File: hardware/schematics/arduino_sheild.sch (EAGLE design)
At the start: 37 parts, among them IC3 LM358, Q1 IRL520N-H, Q2 IRL520N-H, Q3 IRF9Z24, Q4 IRL520N-H, Q5 IRL520N-H, Q6 IRF9Z24, X5 STEREOJACK, X6 STEREOJACK

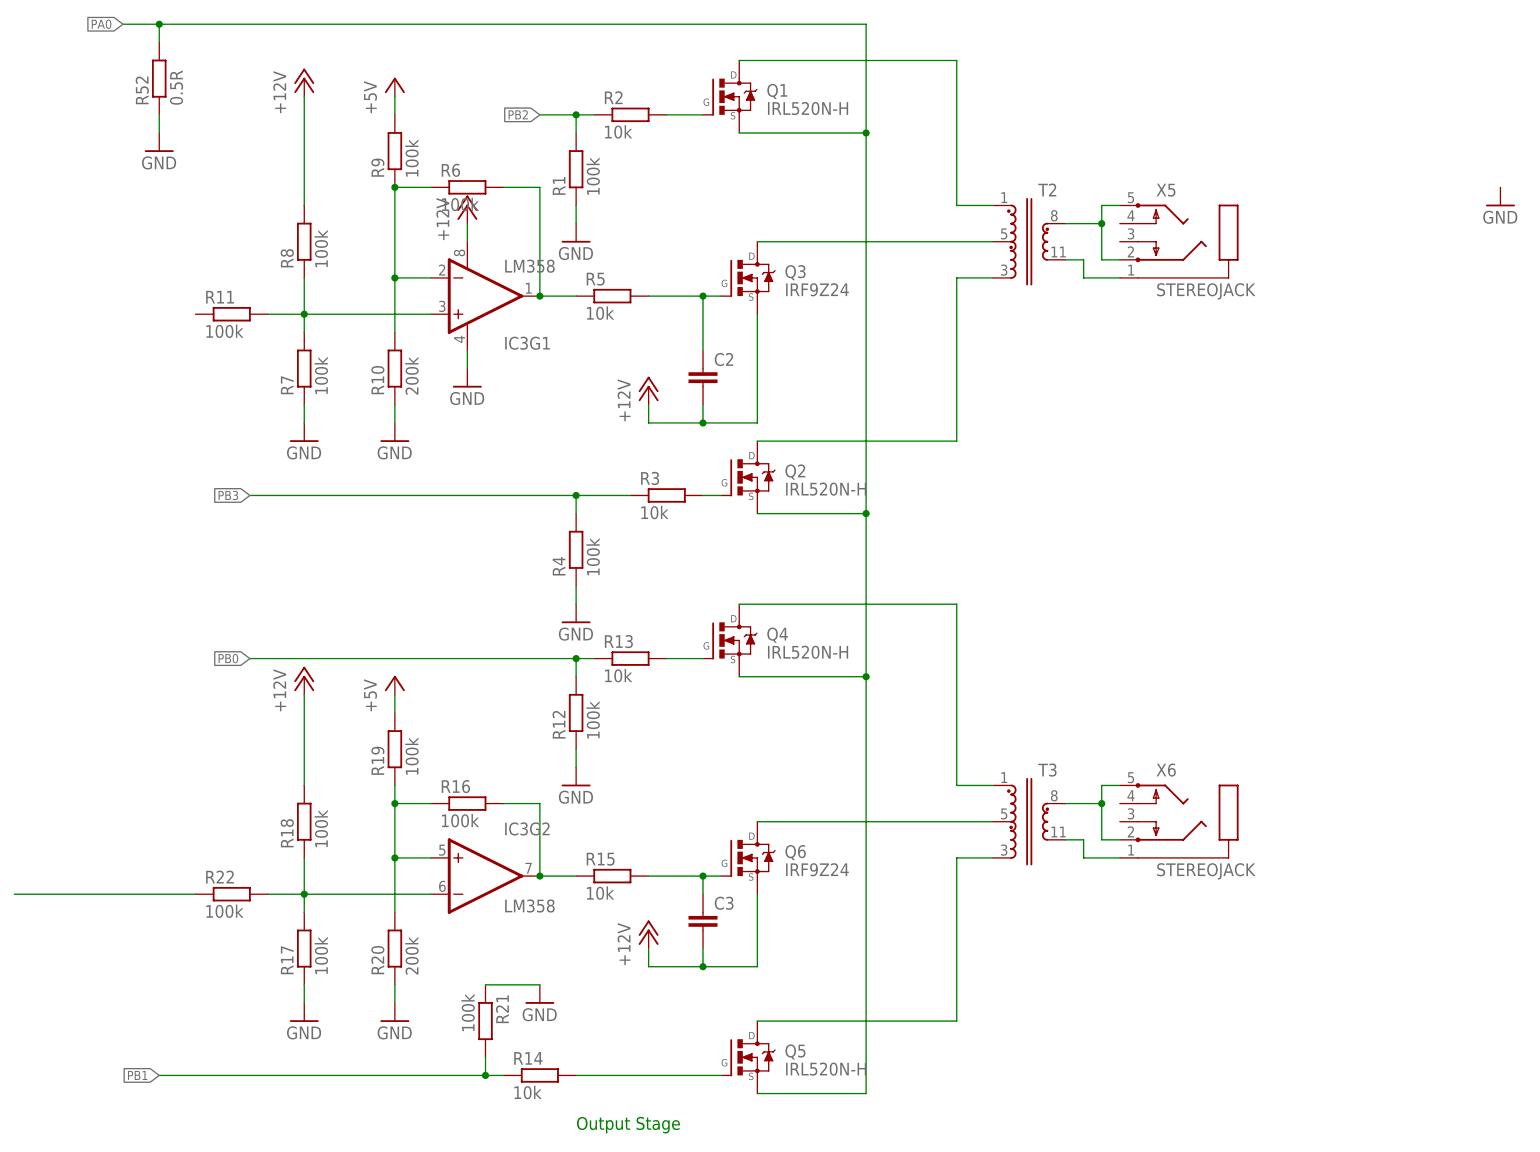
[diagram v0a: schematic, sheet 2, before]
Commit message: Schematics
WIP
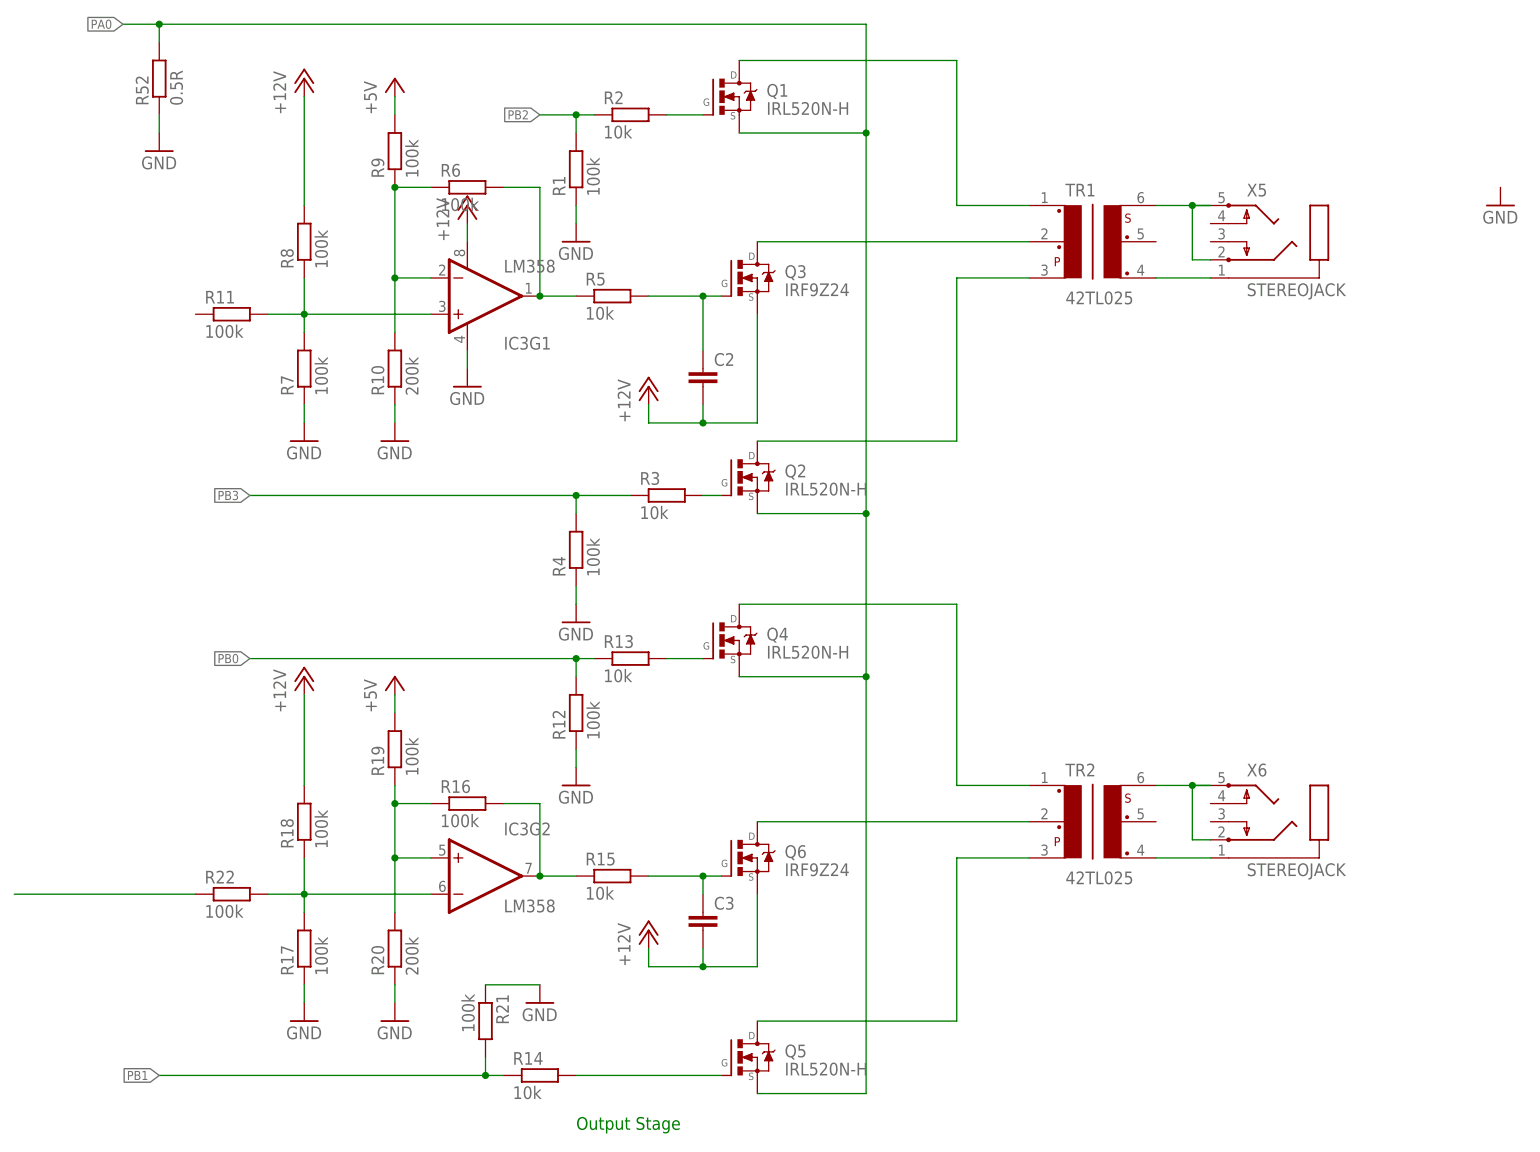
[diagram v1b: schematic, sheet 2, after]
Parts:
- removed T2, T3: (no value), Eagle_POWER_MAGNETICS_rev16b:WE-FB_LT35XX/LT3748_EFD25_750310988
- added TR1, TR2: 42TL025, trafo-xicon:42TL025
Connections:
- removed net N$66: T3.3, X6.1
- removed net N$67: T3.2, X6.2, X6.5
- removed net N$77: T2.3, X5.1
- removed net N$78: T2.2, X5.2, X5.5
- new net N$1: TR1.4, X5.1
- new net N$2: TR1.6, X5.2, X5.5
- new net N$3: TR2.6, X6.2, X6.5
- new net N$4: TR2.4, X6.1
- net N$34: now also TR1.1; no longer T2.1
- net N$35: now also TR1.2; no longer T2.5
- net N$36: now also TR2.1; no longer T3.1
- net N$37: now also TR2.2; no longer T3.5
- net N$38: now also TR2.3; no longer T3.4
- net N$39: now also TR1.3; no longer T2.4
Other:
- moved on the sheet: X5, X6
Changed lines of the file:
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@@
 <part name="R52" library="eagle-ltspice" deviceset="R" device="0207/10" value="0.5R"/>
 <part name="GND21" library="supply1" deviceset="GND" device=""/>
-<part name="T2" library="Eagle_POWER_MAGNETICS_rev16b" deviceset="WE-FB_LT35XX/LT3748_EFD25_750310988" device=""/>
-<part name="T3" library="Eagle_POWER_MAGNETICS_rev16b" deviceset="WE-FB_LT35XX/LT3748_EFD25_750310988" device=""/>
 <part name="U$3" library="adafruit" deviceset="ARDUINO" device="UNO"/>
 <part name="GND40" library="supply1" deviceset="GND" device=""/>
@@
 <part name="P+8" library="supply1" deviceset="+12V" device=""/>
 <part name="P+9" library="supply1" deviceset="+12V" device=""/>
+<part name="TR1" library="trafo-xicon" deviceset="42T?*" device="L" technology="025"/>
+<part name="TR2" library="trafo-xicon" deviceset="42T?*" device="L" technology="025"/>
 </parts>
 <sheets>
@@
 <instance part="R22" gate="G$1" x="50.8" y="40.64"/>
 <instance part="FRAME6" gate="G$1" x="0" y="0"/>
-<instance part="X5" gate="1" x="187.96" y="134.62"/>
-<instance part="X6" gate="1" x="187.96" y="53.34"/>
+<instance part="X5" gate="1" x="200.66" y="134.62"/>
+<instance part="X6" gate="1" x="200.66" y="53.34"/>
 <instance part="R52" gate="G$1" x="40.64" y="154.94" rot="R90"/>
 <instance part="GND21" gate="1" x="40.64" y="144.78"/>
-<instance part="T2" gate="G$1" x="162.56" y="132.08"/>
-<instance part="T3" gate="G$1" x="162.56" y="50.8"/>
 <instance part="GND42" gate="1" x="228.6" y="137.16"/>
 <instance part="P+7" gate="1" x="73.66" y="71.12"/>
@@
 <instance part="P+8" gate="1" x="109.22" y="111.76"/>
 <instance part="P+9" gate="1" x="109.22" y="35.56"/>
+<instance part="TR1" gate="G$1" x="170.18" y="132.08"/>
+<instance part="TR2" gate="G$1" x="170.18" y="50.8"/>
 </instances>
 <busses>
@@
 <wire x1="121.92" y1="157.48" x2="152.4" y2="157.48" width="0.1524" layer="91"/>
 <wire x1="152.4" y1="157.48" x2="152.4" y2="137.16" width="0.1524" layer="91"/>
-<wire x1="157.48" y1="137.16" x2="152.4" y2="137.16" width="0.1524" layer="91"/>
-<pinref part="T2" gate="G$1" pin="1"/>
+<pinref part="TR1" gate="G$1" pin="1"/>
+<wire x1="162.56" y1="137.16" x2="152.4" y2="137.16" width="0.1524" layer="91"/>
 </segment>
 </net>
@@
 <segment>
 <pinref part="Q3" gate="G$1" pin="D"/>
-<wire x1="124.46" y1="132.08" x2="157.48" y2="132.08" width="0.1524" layer="91"/>
-<pinref part="T2" gate="G$1" pin="5"/>
+<wire x1="124.46" y1="132.08" x2="162.56" y2="132.08" width="0.1524" layer="91"/>
+<pinref part="TR1" gate="G$1" pin="2"/>
 </segment>
 </net>
@@
 <wire x1="121.92" y1="81.28" x2="152.4" y2="81.28" width="0.1524" layer="91"/>
 <wire x1="152.4" y1="81.28" x2="152.4" y2="55.88" width="0.1524" layer="91"/>
-<wire x1="157.48" y1="55.88" x2="152.4" y2="55.88" width="0.1524" layer="91"/>
-<pinref part="T3" gate="G$1" pin="1"/>
+<pinref part="TR2" gate="G$1" pin="1"/>
+<wire x1="162.56" y1="55.88" x2="152.4" y2="55.88" width="0.1524" layer="91"/>
 </segment>
 </net>
@@
 <segment>
 <pinref part="Q6" gate="G$1" pin="D"/>
-<wire x1="124.46" y1="50.8" x2="157.48" y2="50.8" width="0.1524" layer="91"/>
-<pinref part="T3" gate="G$1" pin="5"/>
+<wire x1="124.46" y1="50.8" x2="162.56" y2="50.8" width="0.1524" layer="91"/>
+<pinref part="TR2" gate="G$1" pin="2"/>
 </segment>
 </net>
@@
 <wire x1="124.46" y1="22.86" x2="152.4" y2="22.86" width="0.1524" layer="91"/>
 <wire x1="152.4" y1="22.86" x2="152.4" y2="45.72" width="0.1524" layer="91"/>
-<wire x1="157.48" y1="45.72" x2="152.4" y2="45.72" width="0.1524" layer="91"/>
-<pinref part="T3" gate="G$1" pin="4"/>
+<pinref part="TR2" gate="G$1" pin="3"/>
+<wire x1="162.56" y1="45.72" x2="152.4" y2="45.72" width="0.1524" layer="91"/>
 </segment>
 </net>
@@
 <wire x1="124.46" y1="104.14" x2="152.4" y2="104.14" width="0.1524" layer="91"/>
 <wire x1="152.4" y1="104.14" x2="152.4" y2="127" width="0.1524" layer="91"/>
-<wire x1="157.48" y1="127" x2="152.4" y2="127" width="0.1524" layer="91"/>
-<pinref part="T2" gate="G$1" pin="4"/>
+<pinref part="TR1" gate="G$1" pin="3"/>
+<wire x1="162.56" y1="127" x2="152.4" y2="127" width="0.1524" layer="91"/>
 </segment>
 </net>
@@
 </segment>
 </net>
-<net name="N$66" class="0">
-<segment>
-<pinref part="X6" gate="1" pin="1"/>
-<wire x1="175.26" y1="45.72" x2="170.18" y2="45.72" width="0.1524" layer="91"/>
-<wire x1="170.18" y1="45.72" x2="170.18" y2="48.26" width="0.1524" layer="91"/>
-<wire x1="170.18" y1="48.26" x2="167.64" y2="48.26" width="0.1524" layer="91"/>
-<pinref part="T3" gate="G$1" pin="3"/>
-</segment>
-</net>
-<net name="N$67" class="0">
-<segment>
-<pinref part="X6" gate="1" pin="5"/>
-<wire x1="175.26" y1="55.88" x2="172.72" y2="55.88" width="0.1524" layer="91"/>
-<pinref part="X6" gate="1" pin="2"/>
-<wire x1="172.72" y1="55.88" x2="172.72" y2="53.34" width="0.1524" layer="91"/>
-<wire x1="172.72" y1="53.34" x2="172.72" y2="48.26" width="0.1524" layer="91"/>
-<wire x1="172.72" y1="48.26" x2="175.26" y2="48.26" width="0.1524" layer="91"/>
-<pinref part="T3" gate="G$1" pin="2"/>
-<wire x1="167.64" y1="53.34" x2="172.72" y2="53.34" width="0.1524" layer="91"/>
-<junction x="172.72" y="53.34"/>
-</segment>
-</net>
-<net name="N$77" class="0">
-<segment>
-<pinref part="X5" gate="1" pin="1"/>
-<wire x1="175.26" y1="127" x2="170.18" y2="127" width="0.1524" layer="91"/>
-<wire x1="170.18" y1="127" x2="170.18" y2="129.54" width="0.1524" layer="91"/>
-<wire x1="170.18" y1="129.54" x2="167.64" y2="129.54" width="0.1524" layer="91"/>
-<pinref part="T2" gate="G$1" pin="3"/>
-</segment>
-</net>
-<net name="N$78" class="0">
-<segment>
-<pinref part="X5" gate="1" pin="5"/>
-<wire x1="175.26" y1="137.16" x2="172.72" y2="137.16" width="0.1524" layer="91"/>
-<pinref part="X5" gate="1" pin="2"/>
-<wire x1="172.72" y1="137.16" x2="172.72" y2="134.62" width="0.1524" layer="91"/>
-<wire x1="172.72" y1="134.62" x2="172.72" y2="129.54" width="0.1524" layer="91"/>
-<wire x1="172.72" y1="129.54" x2="175.26" y2="129.54" width="0.1524" layer="91"/>
-<pinref part="T2" gate="G$1" pin="2"/>
-<wire x1="167.64" y1="134.62" x2="172.72" y2="134.62" width="0.1524" layer="91"/>
-<junction x="172.72" y="134.62"/>
-</segment>
-</net>
 <net name="PB2" class="0">
 <segment>
@@
 </segment>
 </net>
+<net name="N$1" class="0">
+<segment>
+<pinref part="TR1" gate="G$1" pin="4"/>
+<pinref part="X5" gate="1" pin="1"/>
+<wire x1="180.34" y1="127" x2="187.96" y2="127" width="0.1524" layer="91"/>
+</segment>
+</net>
+<net name="N$2" class="0">
+<segment>
+<pinref part="TR1" gate="G$1" pin="6"/>
+<pinref part="X5" gate="1" pin="5"/>
+<wire x1="180.34" y1="137.16" x2="185.42" y2="137.16" width="0.1524" layer="91"/>
+<wire x1="185.42" y1="137.16" x2="187.96" y2="137.16" width="0.1524" layer="91"/>
+<wire x1="187.96" y1="137.16" x2="185.42" y2="137.16" width="0.1524" layer="91"/>
+<wire x1="185.42" y1="137.16" x2="185.42" y2="129.54" width="0.1524" layer="91"/>
+<pinref part="X5" gate="1" pin="2"/>
+<wire x1="185.42" y1="129.54" x2="187.96" y2="129.54" width="0.1524" layer="91"/>
+<junction x="185.42" y="137.16"/>
+</segment>
+</net>
+<net name="N$3" class="0">
+<segment>
+<pinref part="TR2" gate="G$1" pin="6"/>
+<pinref part="X6" gate="1" pin="5"/>
+<wire x1="180.34" y1="55.88" x2="185.42" y2="55.88" width="0.1524" layer="91"/>
+<wire x1="185.42" y1="55.88" x2="187.96" y2="55.88" width="0.1524" layer="91"/>
+<wire x1="187.96" y1="55.88" x2="185.42" y2="55.88" width="0.1524" layer="91"/>
+<wire x1="185.42" y1="55.88" x2="185.42" y2="48.26" width="0.1524" layer="91"/>
+<pinref part="X6" gate="1" pin="2"/>
+<wire x1="185.42" y1="48.26" x2="187.96" y2="48.26" width="0.1524" layer="91"/>
+<junction x="185.42" y="55.88"/>
+</segment>
+</net>
+<net name="N$4" class="0">
+<segment>
+<pinref part="X6" gate="1" pin="1"/>
+<pinref part="TR2" gate="G$1" pin="4"/>
+<wire x1="187.96" y1="45.72" x2="180.34" y2="45.72" width="0.1524" layer="91"/>
+</segment>
+</net>
